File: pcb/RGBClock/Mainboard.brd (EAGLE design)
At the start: 99.8 x 70.1 mm, 102 parts, among them IC1 MCP23017SO, IC2 LT1763CS8-1.5, K1 G6K-2F, K2 G6K-2F, K3 G6K-2F, K4 G6K-2F, Q1 32.768KHz, U1 MAX6369KA+T, U10 NX3L1G384GW, U11 NX3L1G384GW, U13 DRV612PW, U14 2N7002-7-F, U15 2N7002-7-F, U16 2N7002-7-F, U17 2N7002-7-F, U2 TXS0102DCUR, U3 P82B96DR, U4 LM2675M-5.0, U5 DS1338Z-33+, U7 TPS71533DCKR, U8 NX3L1G384GW, U9 NX3L1G384GW, X2 43045-0400, X3 CON-LUMBERG_1503_09, X4 CON-LUMBERG_1503_09, X5 43045-0800, X6 ST-SMB-H

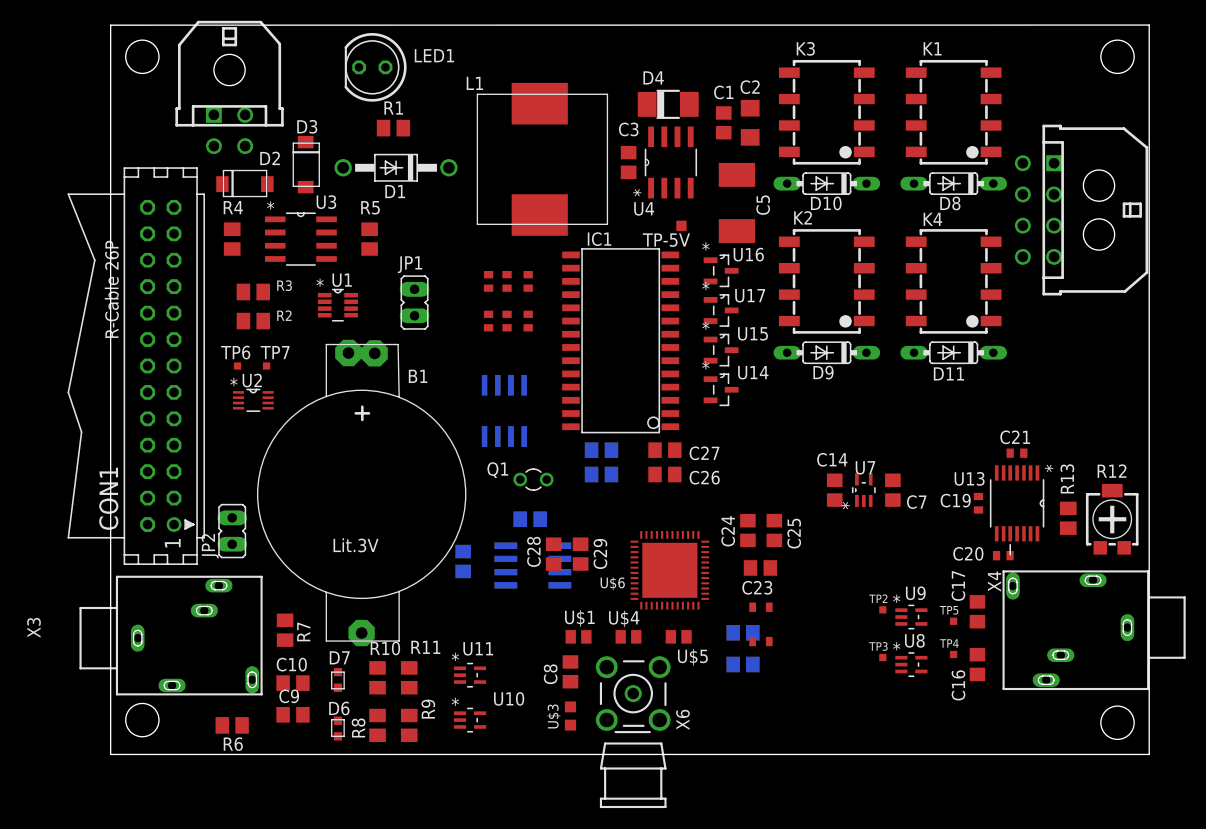
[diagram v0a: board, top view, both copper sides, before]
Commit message: routed
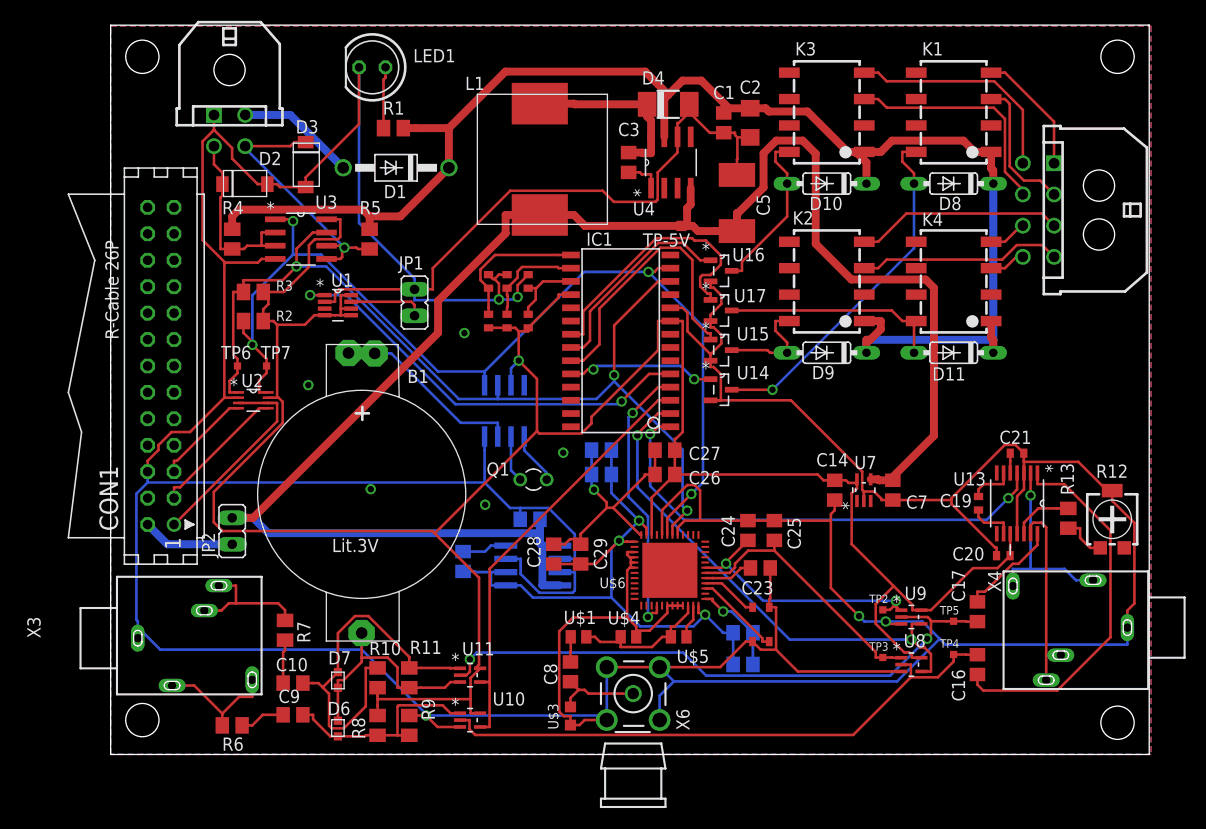
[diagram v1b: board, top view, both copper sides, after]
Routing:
- net GND: track 0.00 -> 614.4 mm, vias 0 -> 10
- net +3V3: track 0.00 -> 243.0 mm, vias 0 -> 1
- net +5V: track 0.00 -> 166.7 mm
- net VCC: track 0.00 -> 143.6 mm
- net SDA: track 0.00 -> 99.5 mm, vias 0 -> 4
- net SCL: track 0.00 -> 92.6 mm, vias 0 -> 3
- net +1.8V: track 0.00 -> 62.8 mm, vias 0 -> 3
- net N$30: track 0.00 -> 58.3 mm, vias 0 -> 2
- net N$29: track 0.00 -> 56.6 mm
- net N$66: track 0.00 -> 49.0 mm, vias 0 -> 2
- net N$38: track 0.00 -> 46.6 mm, vias 0 -> 2
- net N$33: track 0.00 -> 41.6 mm, vias 0 -> 2
- net N$31: track 0.00 -> 41.1 mm
- net N$53: track 0.00 -> 36.3 mm
- net N$36: track 0.00 -> 36.3 mm
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- added copper zone on layer 1, net GND
- added copper zone on layer 16, net GND
